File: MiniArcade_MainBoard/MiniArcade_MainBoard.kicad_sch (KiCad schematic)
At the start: 30 parts, among them J1 62701021721, J2 Conn_01x05_Pin, J3 Conn_01x06_Pin, J4 F3311A7H121026E200, SW1 EVPAA, U1 ATSAMD21J18A-A, U2 LM321

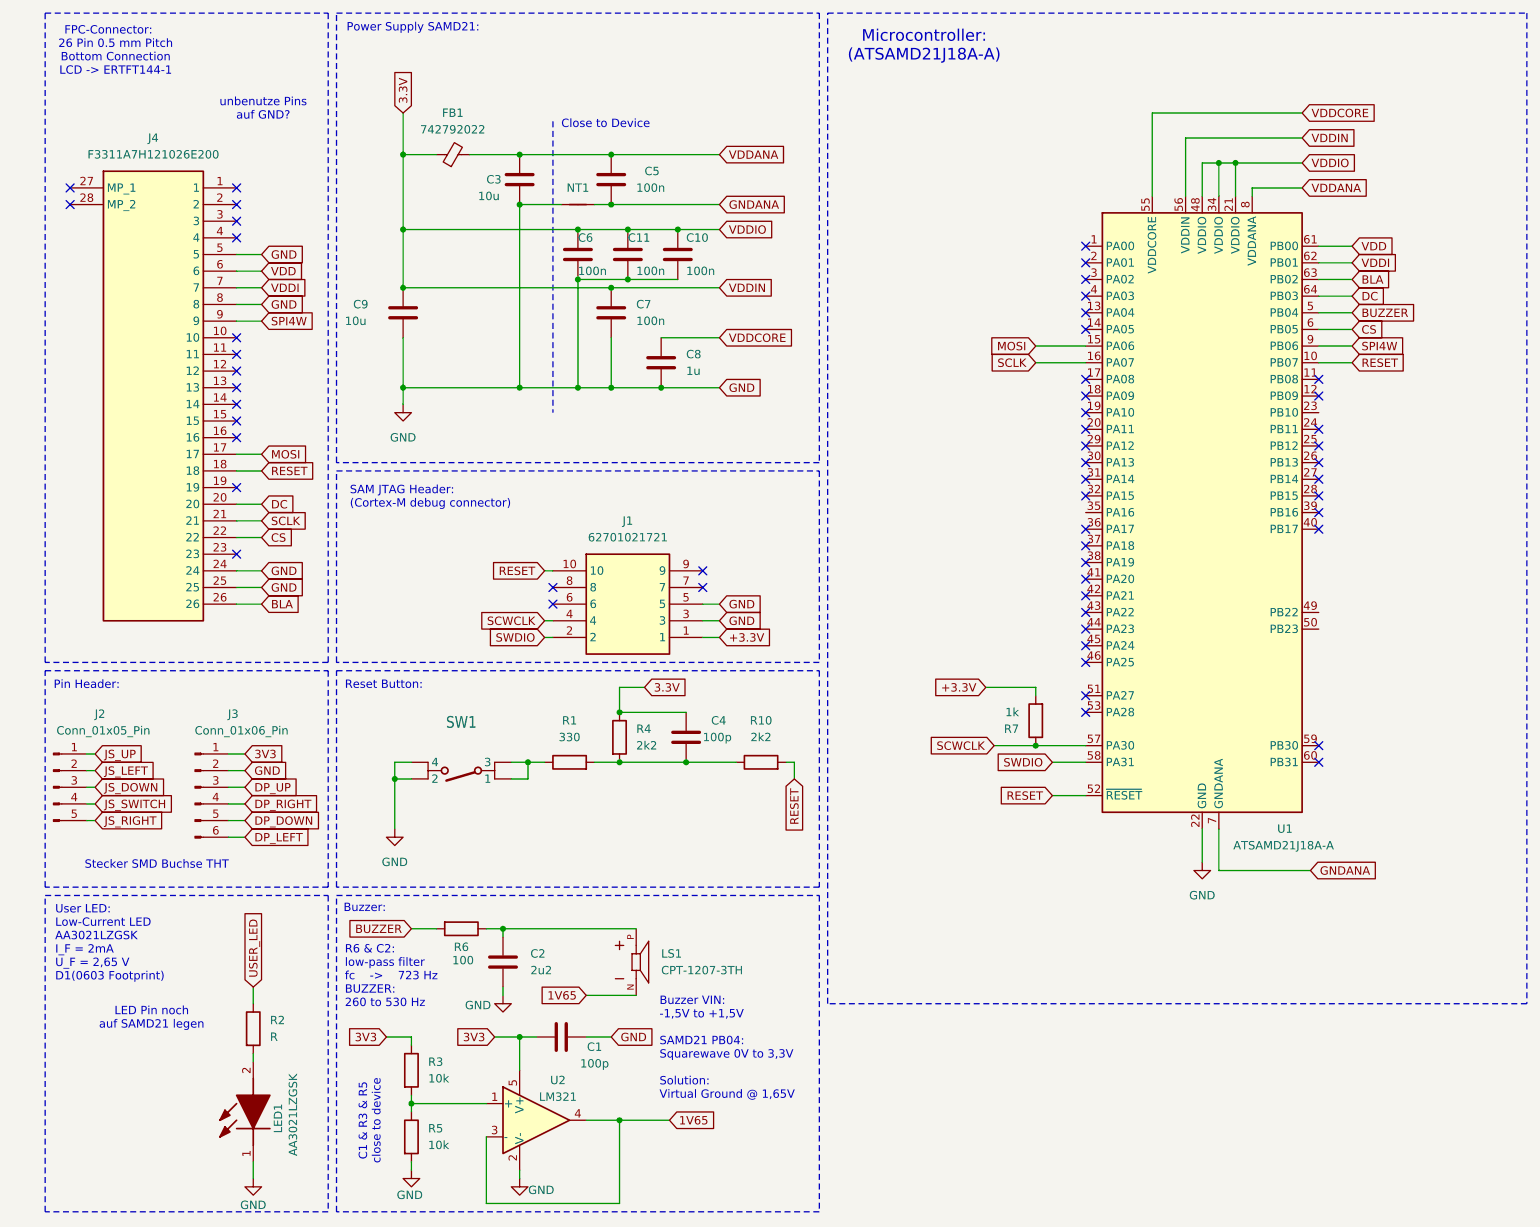
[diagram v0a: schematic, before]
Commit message: stand 03 11
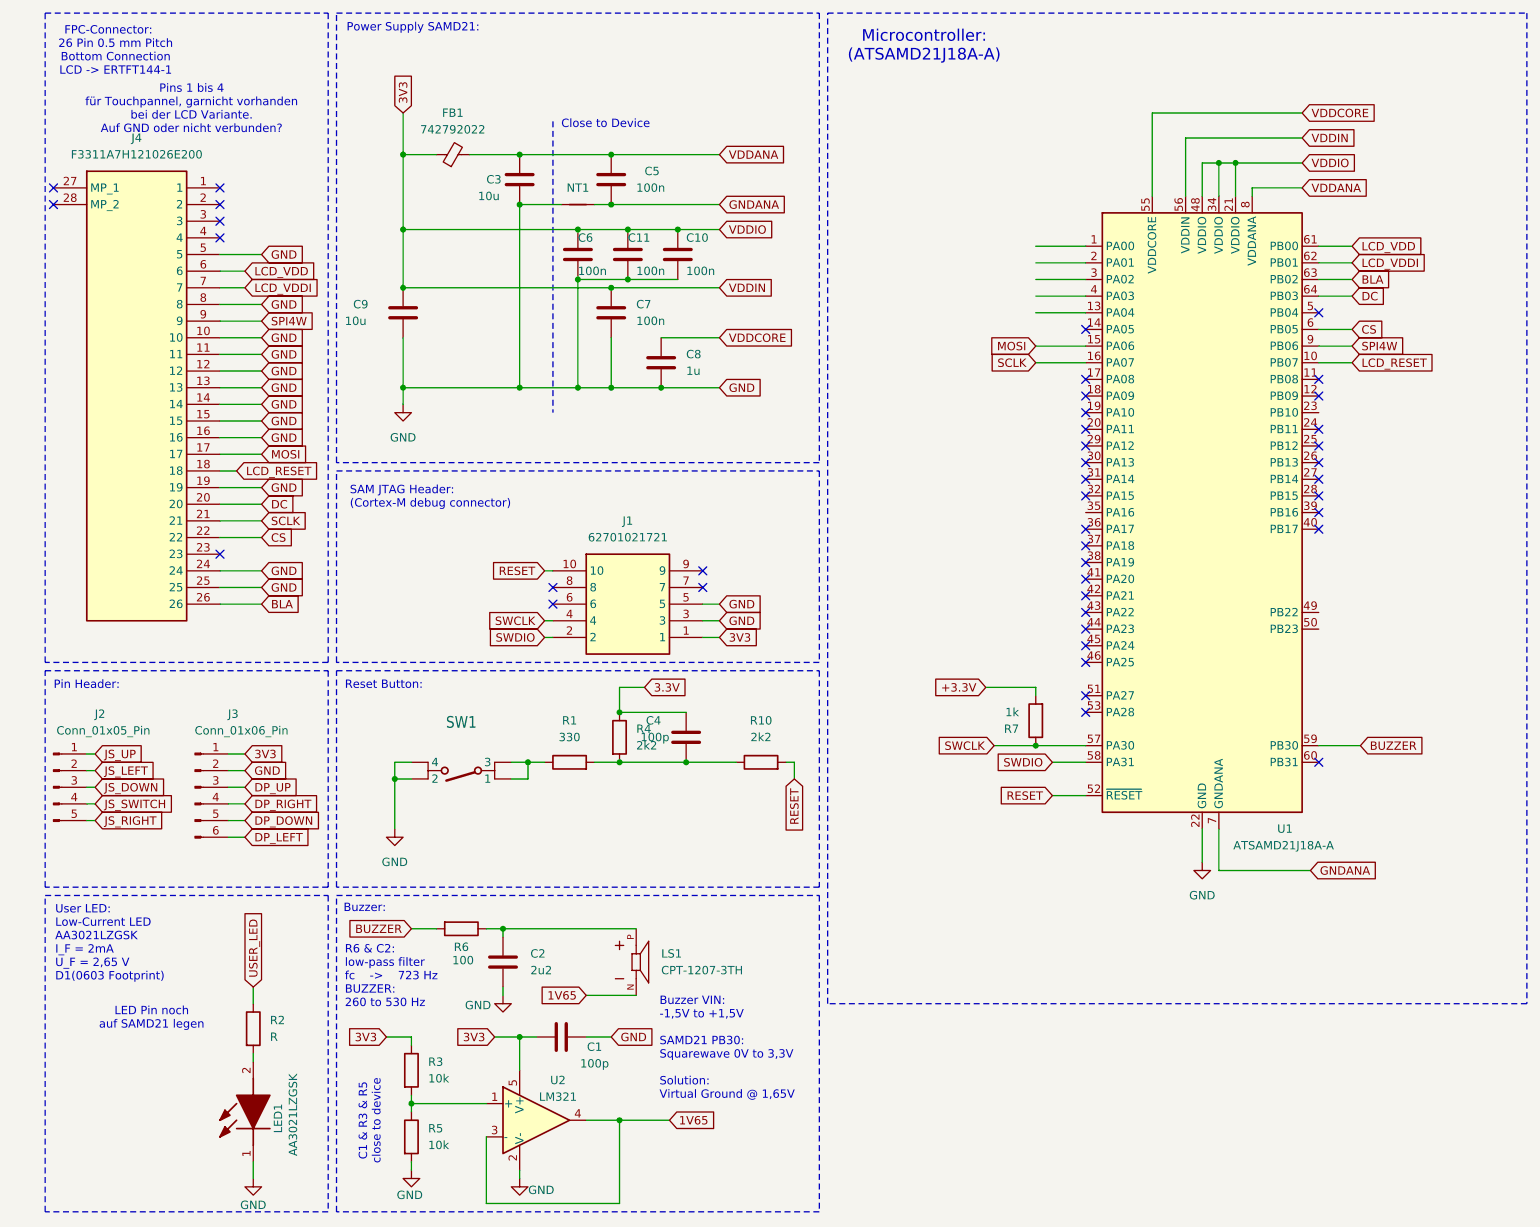
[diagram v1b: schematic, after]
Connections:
- net +3.3V: no longer J1.1
- net 3.3V: no longer C10.1, C11.1, C6.1, C7.1, C9.1, FB1.1, U1.21 (VDDIO), U1.34 (VDDIO), U1.48 (VDDIO), U1.56 (VDDIN)
- net 3V3: now also C10.1, C11.1, C6.1, C7.1, C9.1, FB1.1, J1.1, U1.21 (VDDIO), U1.34 (VDDIO), U1.48 (VDDIO), U1.56 (VDDIN)
- net BUZZER: now also U1.59 (PB30); no longer U1.5 (PB04)
- net GND: now also J4.10, J4.11, J4.12, J4.13, J4.14, J4.15, J4.16, J4.19
- net RESET: no longer J4.18, U1.10 (PB07)
- net SCWCLK renamed SWCLK
- net VDD renamed LCD_VDD
- net VDDI renamed LCD_VDDI
- new net LCD_RESET: J4.18, U1.10 (PB07)
- no-connect marks 55 -> 42
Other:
- note added: "Buzzer VIN: -1,5V to +1,5V SAMD21 PB30: Squarewave 0V to 3,3V Solution: Virtual Ground @ 1,65V"
- note added: "Pins 1 bis 4 für Touchpannel, garnicht vorhanden bei der LCD Variante. Auf GND oder nicht verbunden?"
- note removed: "Buzzer VIN: -1,5V to +1,5V SAMD21 PB04: Squarewave 0V to 3,3V Solution: Virtual Ground @ 1,65V"
- note removed: "Stecker SMD Buchse THT"
- note removed: "unbenutze Pins auf GND?"
- moved on the sheet: J4

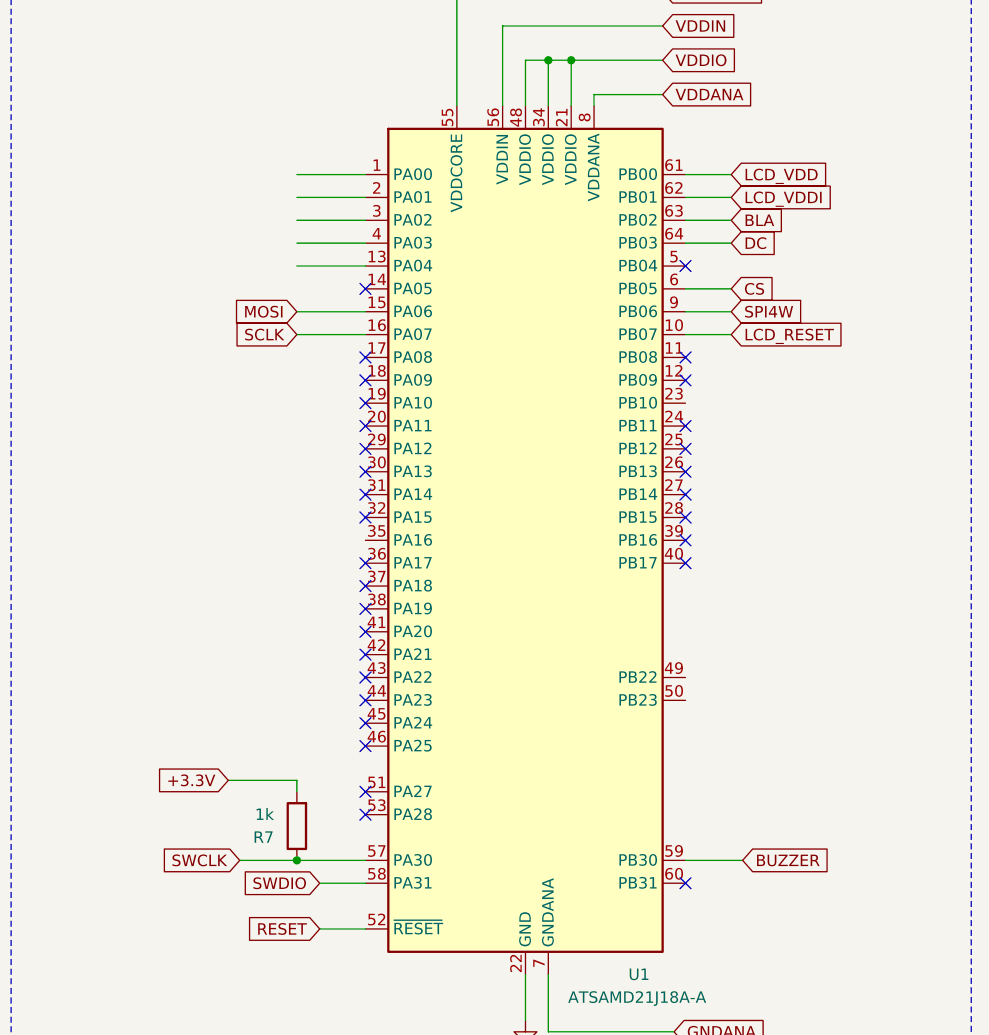
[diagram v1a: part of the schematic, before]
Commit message: stand 04 11 2025
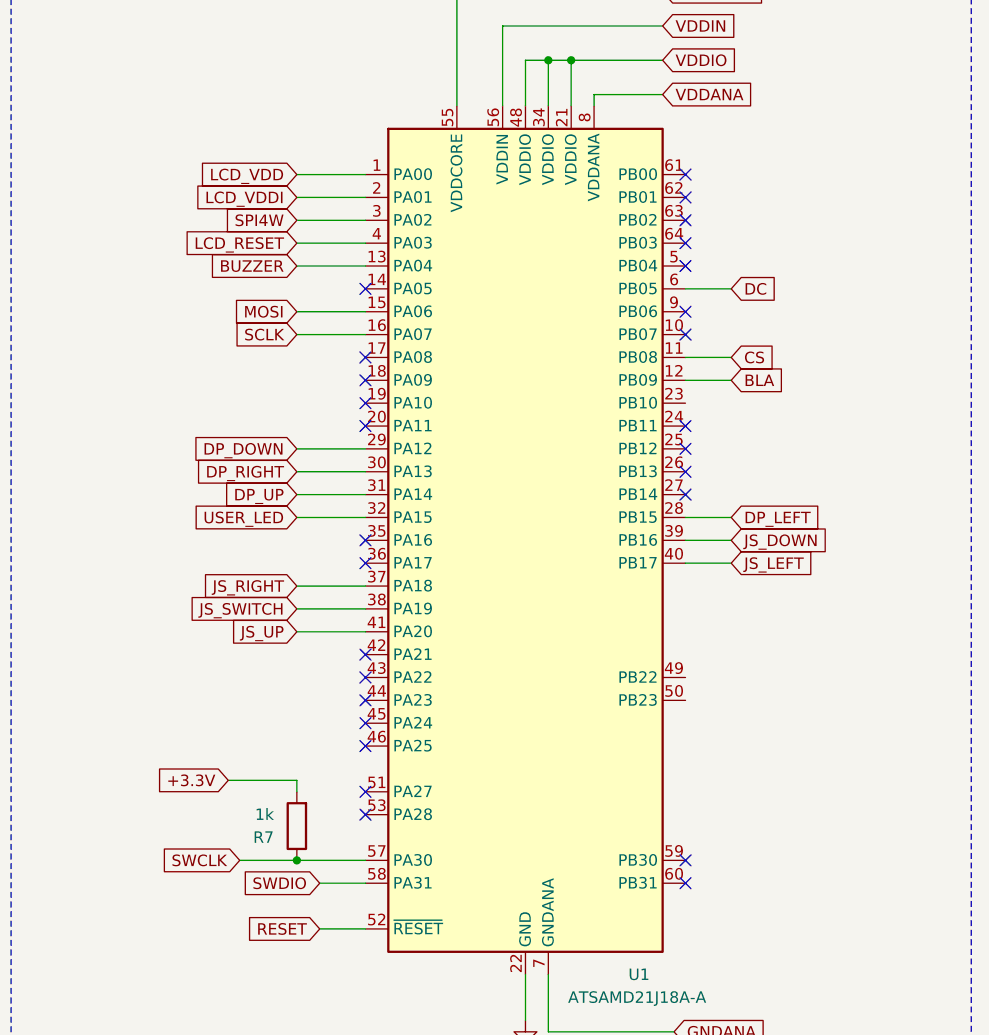
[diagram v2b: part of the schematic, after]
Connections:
- net BLA: now also U1.12 (PB09); no longer U1.63 (PB02)
- net BUZZER: now also U1.13 (PA04); no longer U1.59 (PB30)
- net CS: now also U1.11 (PB08); no longer U1.6 (PB05)
- net DC: now also U1.6 (PB05); no longer U1.64 (PB03)
- net DP_DOWN: now also U1.29 (PA12)
- net DP_LEFT: now also U1.28 (PB15)
- net DP_RIGHT: now also U1.30 (PA13)
- net DP_UP: now also U1.31 (PA14)
- net JS_DOWN: now also U1.39 (PB16)
- net JS_LEFT: now also U1.40 (PB17)
- net JS_RIGHT: now also U1.37 (PA18)
- net JS_SWITCH: now also U1.38 (PA19)
- net JS_UP: now also U1.41 (PA20)
- net LCD_RESET: now also U1.4 (PA03); no longer U1.10 (PB07)
- net LCD_VDD: now also U1.1 (PA00); no longer U1.61 (PB00)
- net LCD_VDDI: now also U1.2 (PA01); no longer U1.62 (PB01)
- net SPI4W: now also U1.3 (PA02); no longer U1.9 (PB06)
- net USER_LED: now also U1.32 (PA15)
- no-connect marks 42 -> 38
